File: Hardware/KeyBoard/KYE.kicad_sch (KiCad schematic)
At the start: 121 parts

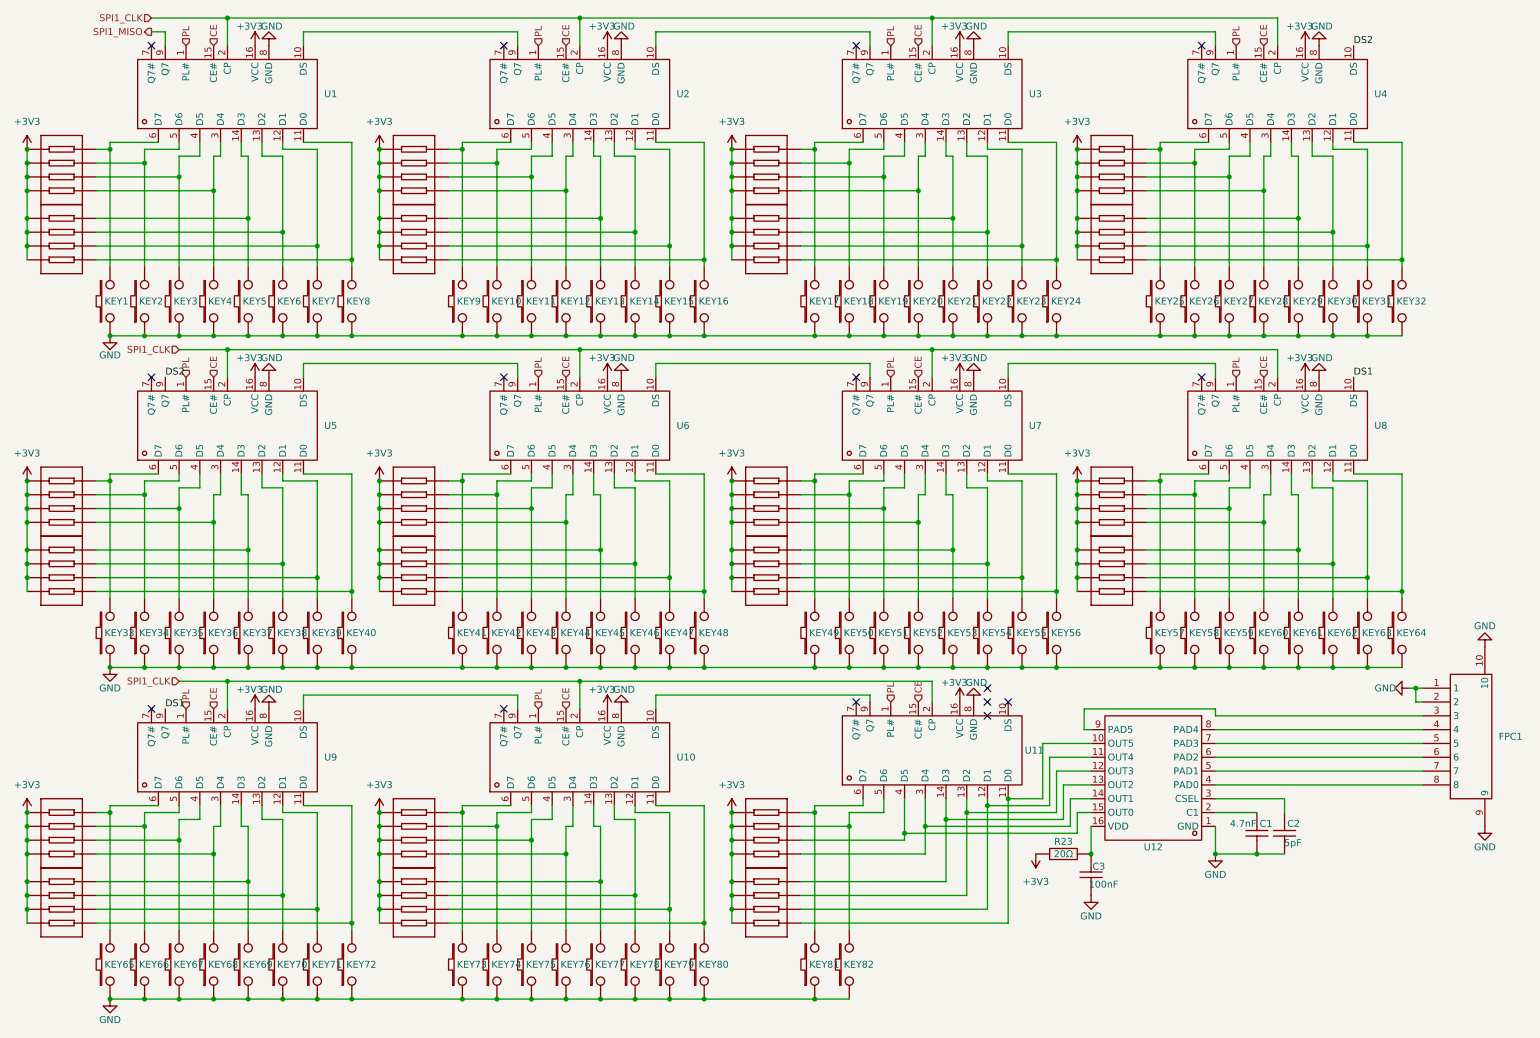
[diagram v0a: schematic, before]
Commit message: complete all
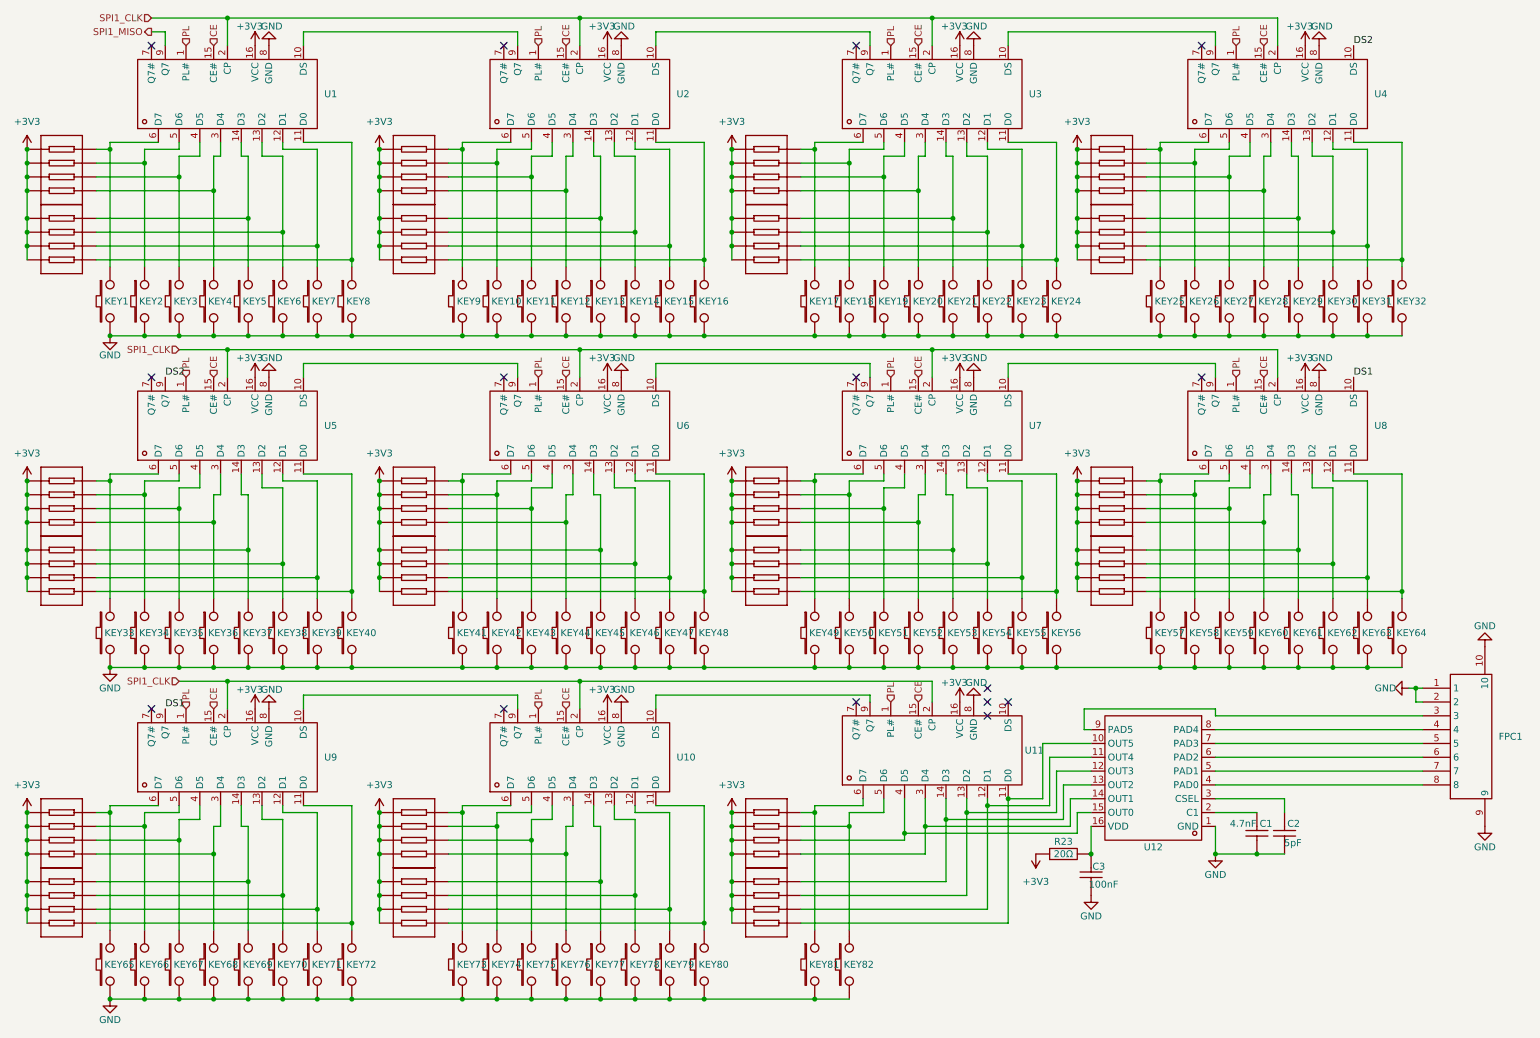
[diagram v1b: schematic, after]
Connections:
- net GND: now also KEY1.2, KEY10.2, KEY11.2, KEY12.2, KEY13.2, KEY14.2, KEY15.2, KEY16.2, KEY17.2, KEY18.2, KEY19.2, KEY2.2, KEY20.2, KEY21.2, KEY22.2, KEY23.2, KEY24.2, KEY25.2, KEY26.2, KEY27.2, KEY28.2, KEY29.2, KEY3.2, KEY30.2, KEY31.2, KEY32.2, KEY33.2, KEY34.2, KEY35.2, KEY36.2, KEY37.2, KEY38.2, KEY39.2, KEY4.2, KEY40.2, KEY41.2, KEY42.2, KEY43.2, KEY44.2, KEY45.2, KEY46.2, KEY47.2, KEY48.2, KEY49.2, KEY5.2, KEY50.2, KEY51.2, KEY52.2, KEY53.2, KEY54.2, KEY55.2, KEY56.2, KEY57.2, KEY58.2, KEY59.2, KEY6.2, KEY60.2, KEY61.2, KEY62.2, KEY63.2, KEY64.2, KEY65.2, KEY66.2, KEY67.2, KEY68.2, KEY69.2, KEY7.2, KEY70.2, KEY71.2, KEY72.2, KEY73.2, KEY74.2, KEY75.2, KEY76.2, KEY77.2, KEY78.2, KEY79.2, KEY8.2, KEY80.2, KEY81.2, KEY82.2, KEY9.2; no longer KEY1.1, KEY10.1, KEY11.1, KEY12.1, KEY13.1, KEY14.1, KEY15.1, KEY16.1, KEY17.1, KEY18.1, KEY19.1, KEY2.1, KEY20.1, KEY21.1, KEY22.1, KEY23.1, KEY24.1, KEY25.1, KEY26.1, KEY27.1, KEY28.1, KEY29.1, KEY3.1, KEY30.1, KEY31.1, KEY32.1, KEY33.1, KEY34.1, KEY35.1, KEY36.1, KEY37.1, KEY38.1, KEY39.1, KEY4.1, KEY40.1, KEY41.1, KEY42.1, KEY43.1, KEY44.1, KEY45.1, KEY46.1, KEY47.1, KEY48.1, KEY49.1, KEY5.1, KEY50.1, KEY51.1, KEY52.1, KEY53.1, KEY54.1, KEY55.1, KEY56.1, KEY57.1, KEY58.1, KEY59.1, KEY6.1, KEY60.1, KEY61.1, KEY62.1, KEY63.1, KEY64.1, KEY65.1, KEY66.1, KEY67.1, KEY68.1, KEY69.1, KEY7.1, KEY70.1, KEY71.1, KEY72.1, KEY73.1, KEY74.1, KEY75.1, KEY76.1, KEY77.1, KEY78.1, KEY79.1, KEY8.1, KEY80.1, KEY81.1, KEY82.1, KEY9.1
- net at R4.1, U2.14 (D3): now also KEY13.1; no longer KEY13.2
- net at R4.2, U2.13 (D2): now also KEY14.1; no longer KEY14.2
- net at R4.3, U2.12 (D1): now also KEY15.1; no longer KEY15.2
- net at R4.4, U2.11 (D0): now also KEY16.1; no longer KEY16.2
- net at R15.2, U8.5 (D6): now also KEY58.1; no longer KEY58.2
- net at R9.3, U5.4 (D5): now also KEY35.1; no longer KEY35.2
- net at R16.4, U8.11 (D0): now also KEY64.1; no longer KEY64.2
- net at R2.2, U1.13 (D2): now also KEY6.1; no longer KEY6.2
- net at R14.1, U7.14 (D3): now also KEY53.1; no longer KEY53.2
- net at R12.4, U6.11 (D0): now also KEY48.1; no longer KEY48.2
- net at R9.2, U5.5 (D6): now also KEY34.1; no longer KEY34.2
- net at R3.1, U2.6 (D7): now also KEY9.1; no longer KEY9.2
- net at R5.1, U3.6 (D7): now also KEY17.1; no longer KEY17.2
- net at R17.2, U9.5 (D6): now also KEY66.1; no longer KEY66.2
- net at R21.1, U11.6 (D7): now also KEY81.1; no longer KEY81.2
- net at R21.2, U11.5 (D6): now also KEY82.1; no longer KEY82.2
- net at R19.1, U10.6 (D7): now also KEY73.1; no longer KEY73.2
- net at R19.2, U10.5 (D6): now also KEY74.1; no longer KEY74.2
- net at R19.3, U10.4 (D5): now also KEY75.1; no longer KEY75.2
- net at R19.4, U10.3 (D4): now also KEY76.1; no longer KEY76.2
- net at R8.1, U4.14 (D3): now also KEY29.1; no longer KEY29.2
- net at R12.2, U6.13 (D2): now also KEY46.1; no longer KEY46.2
- net at R18.3, U9.12 (D1): now also KEY71.1; no longer KEY71.2
- net at R14.4, U7.11 (D0): now also KEY56.1; no longer KEY56.2
- net at R14.3, U7.12 (D1): now also KEY55.1; no longer KEY55.2
- net at R14.2, U7.13 (D2): now also KEY54.1; no longer KEY54.2
- net at R13.4, U7.3 (D4): now also KEY52.1; no longer KEY52.2
- net at R13.3, U7.4 (D5): now also KEY51.1; no longer KEY51.2
- net at R13.2, U7.5 (D6): now also KEY50.1; no longer KEY50.2
- net at R13.1, U7.6 (D7): now also KEY49.1; no longer KEY49.2
- net at R9.1, U5.6 (D7): now also KEY33.1; no longer KEY33.2
- net at R9.4, U5.3 (D4): now also KEY36.1; no longer KEY36.2
- net at R20.1, U10.14 (D3): now also KEY77.1; no longer KEY77.2
- net at R20.2, U10.13 (D2): now also KEY78.1; no longer KEY78.2
- net at R20.3, U10.12 (D1): now also KEY79.1; no longer KEY79.2
- net at R20.4, U10.11 (D0): now also KEY80.1; no longer KEY80.2
- net at R3.3, U2.4 (D5): now also KEY11.1; no longer KEY11.2
- net at R6.1, U3.14 (D3): now also KEY21.1; no longer KEY21.2
- net at R1.1, U1.6 (D7): now also KEY1.1; no longer KEY1.2
- net at R16.3, U8.12 (D1): now also KEY63.1; no longer KEY63.2
- net at R10.4, U5.11 (D0): now also KEY40.1; no longer KEY40.2
- net at R10.3, U5.12 (D1): now also KEY39.1; no longer KEY39.2
- net at R10.2, U5.13 (D2): now also KEY38.1; no longer KEY38.2
- net at R10.1, U5.14 (D3): now also KEY37.1; no longer KEY37.2
- net at R7.1, U4.6 (D7): now also KEY25.1; no longer KEY25.2
- net at R18.2, U9.13 (D2): now also KEY70.1; no longer KEY70.2
- net at R18.4, U9.11 (D0): now also KEY72.1; no longer KEY72.2
- net at R12.3, U6.12 (D1): now also KEY47.1; no longer KEY47.2
- net at R16.1, U8.14 (D3): now also KEY61.1; no longer KEY61.2
- net at R18.1, U9.14 (D3): now also KEY69.1; no longer KEY69.2
- net at R17.4, U9.3 (D4): now also KEY68.1; no longer KEY68.2
- net at R17.3, U9.4 (D5): now also KEY67.1; no longer KEY67.2
- net at R17.1, U9.6 (D7): now also KEY65.1; no longer KEY65.2
- net at R2.1, U1.14 (D3): now also KEY5.1; no longer KEY5.2
- net at R2.3, U1.12 (D1): now also KEY7.1; no longer KEY7.2
- net at R2.4, U1.11 (D0): now also KEY8.1; no longer KEY8.2
- net at R3.4, U2.3 (D4): now also KEY12.1; no longer KEY12.2
- net at R15.4, U8.3 (D4): now also KEY60.1; no longer KEY60.2
- net at R1.4, U1.3 (D4): now also KEY4.1; no longer KEY4.2
- net at R1.3, U1.4 (D5): now also KEY3.1; no longer KEY3.2
- net at R1.2, U1.5 (D6): now also KEY2.1; no longer KEY2.2
- net at R6.2, U3.13 (D2): now also KEY22.1; no longer KEY22.2
- net at R6.3, U3.12 (D1): now also KEY23.1; no longer KEY23.2
- net at R11.1, U6.6 (D7): now also KEY41.1; no longer KEY41.2
- net at R15.3, U8.4 (D5): now also KEY59.1; no longer KEY59.2
- net at R8.2, U4.13 (D2): now also KEY30.1; no longer KEY30.2
- net at R15.1, U8.6 (D7): now also KEY57.1; no longer KEY57.2
- net at R11.2, U6.5 (D6): now also KEY42.1; no longer KEY42.2
- net at R8.3, U4.12 (D1): now also KEY31.1; no longer KEY31.2
- net at R11.3, U6.4 (D5): now also KEY43.1; no longer KEY43.2
- net at R11.4, U6.3 (D4): now also KEY44.1; no longer KEY44.2
- net at R12.1, U6.14 (D3): now also KEY45.1; no longer KEY45.2
- net at R16.2, U8.13 (D2): now also KEY62.1; no longer KEY62.2
- net at R7.4, U4.3 (D4): now also KEY28.1; no longer KEY28.2
- net at R3.2, U2.5 (D6): now also KEY10.1; no longer KEY10.2
- net at R8.4, U4.11 (D0): now also KEY32.1; no longer KEY32.2
- net at R7.3, U4.4 (D5): now also KEY27.1; no longer KEY27.2
- net at R7.2, U4.5 (D6): now also KEY26.1; no longer KEY26.2
- net at R5.3, U3.4 (D5): now also KEY19.1; no longer KEY19.2
- net at R5.4, U3.3 (D4): now also KEY20.1; no longer KEY20.2
- net at R6.4, U3.11 (D0): now also KEY24.1; no longer KEY24.2
- net at R5.2, U3.5 (D6): now also KEY18.1; no longer KEY18.2
